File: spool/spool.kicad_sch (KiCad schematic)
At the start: 135 parts, among them J1 USB_B_Micro, J13 Conn_02x10_Counter_Clockwise, J14 Conn_01x07, J2 SWD, J3 Switch_1, J4 Switch_1, J5 Switch_1, J6 Switch_2, J7 Conn_01x02, J8 Conn_01x08, M1 Motor_DC, Q1 AO3400A, Q101 Q_NMOS_GSD, Q2 2N7002, SW1 USB_BOOT, SW2 RESET, SW3 SW_Push_DPDT, SW4 SW_Coded_SH-7010, SW5 SW_Push_DPDT, U1 TPS63070RNMR, U10 HT75xx-1-SOT89, U101 MMA8451QR1, U102 INA219AxDCN, U103 DY-ITR8402, U104 DY-ITR8402, U11 TPL0401B-10-Q1, U12 BS612, U14 PCF8563T, U3 AS5600-ASOT, U6 DRV8871DDA, U7 W25Q128JVS, U8 RP2040, U9 BS612, Y1 Crystal_GND24, Y2 Crystal

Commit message: Tidy up
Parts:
- BT1: now left out of the parts list
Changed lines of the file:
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@@
 		(unit 1)
 		(exclude_from_sim no)
-		(in_bom yes)
+		(in_bom no)
 		(on_board yes)
 		(dnp no)

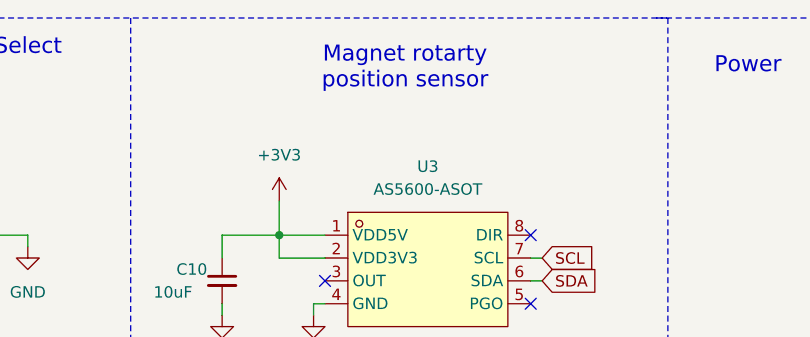
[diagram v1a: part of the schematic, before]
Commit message: Add Readme file
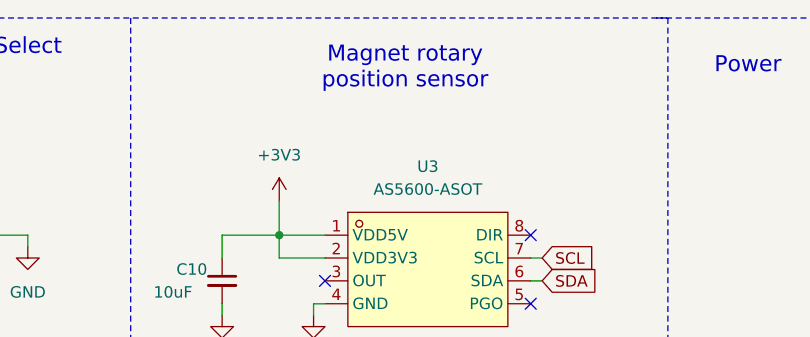
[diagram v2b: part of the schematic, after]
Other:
- note added: "Magnet rotary position sensor"
- note removed: "Magnet rotarty position sensor"
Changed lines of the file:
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@@
 		)
 	)
-	(text "Magnet rotarty \nposition sensor"
+	(text "Magnet rotary \nposition sensor"
 		(exclude_from_sim no)
 		(at 129.54 19.558 0)
